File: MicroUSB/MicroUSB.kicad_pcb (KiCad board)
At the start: 2 copper layers, 21.8 x 9.9 mm, 6 parts, among them J1 USB_B_Micro, J2 Conn_01x05

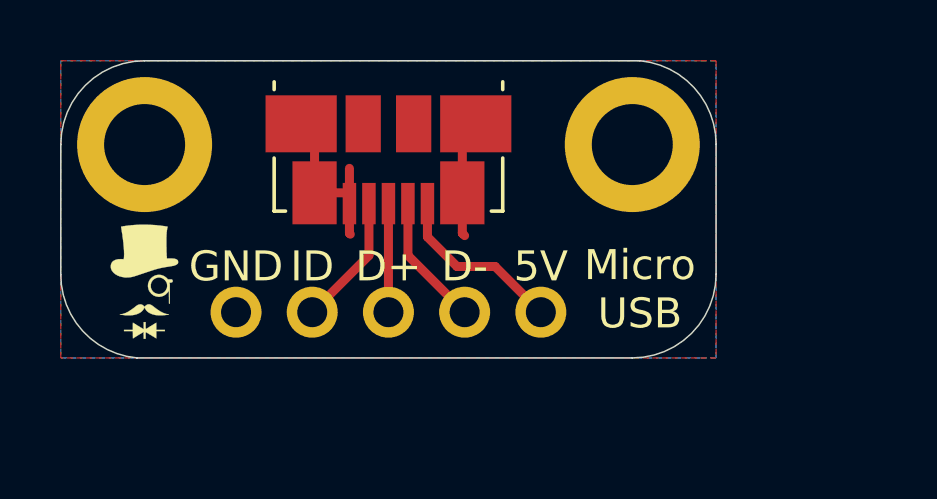
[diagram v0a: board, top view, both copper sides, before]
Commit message: Board Redesign
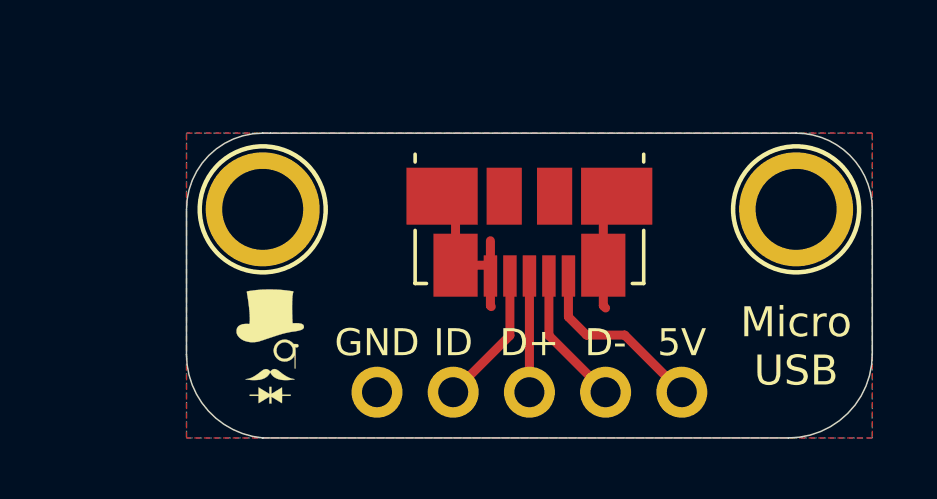
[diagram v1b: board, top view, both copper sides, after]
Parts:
- H1, H2: footprint MountingHole:MountingHole_2.7mm_M2.5_ISO14580_Pad -> SirBoardLibrary:MountingHole_M2.5_SirBoard
- moved H2 21.8 mm to (74.9, 32.4), turned to 0 degrees
- moved H1 12.5 mm to (57.1, 32.4), turned to 0 degrees
- moved J2 5.40 mm to (71.1, 38.5)
- moved G*** 5.28 mm to (66.0, 32.6)
- moved J1 5.28 mm to (66.0, 33.1)
- moved G*** 4.71 mm to (57.4, 37.0)
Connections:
- net Net-(J1-Pad1) renamed /VBus
- net Net-(J1-Pad2) renamed /D-
- net Net-(J1-Pad3) renamed /D+
- net Net-(J1-Pad4) renamed /ID
- net Net-(J1-Pad5) renamed /GND
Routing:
- added copper zone on B.Cu, net /VBus
- removed copper zone on B.Cu, net /GND
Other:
- board size 21.8 x 9.9 mm -> 22.9 x 10.2 mm
